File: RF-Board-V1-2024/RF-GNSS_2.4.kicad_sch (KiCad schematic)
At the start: 11 parts, among them J4 UART, J5 Conn_Coaxial, J7 Conn_Coaxial

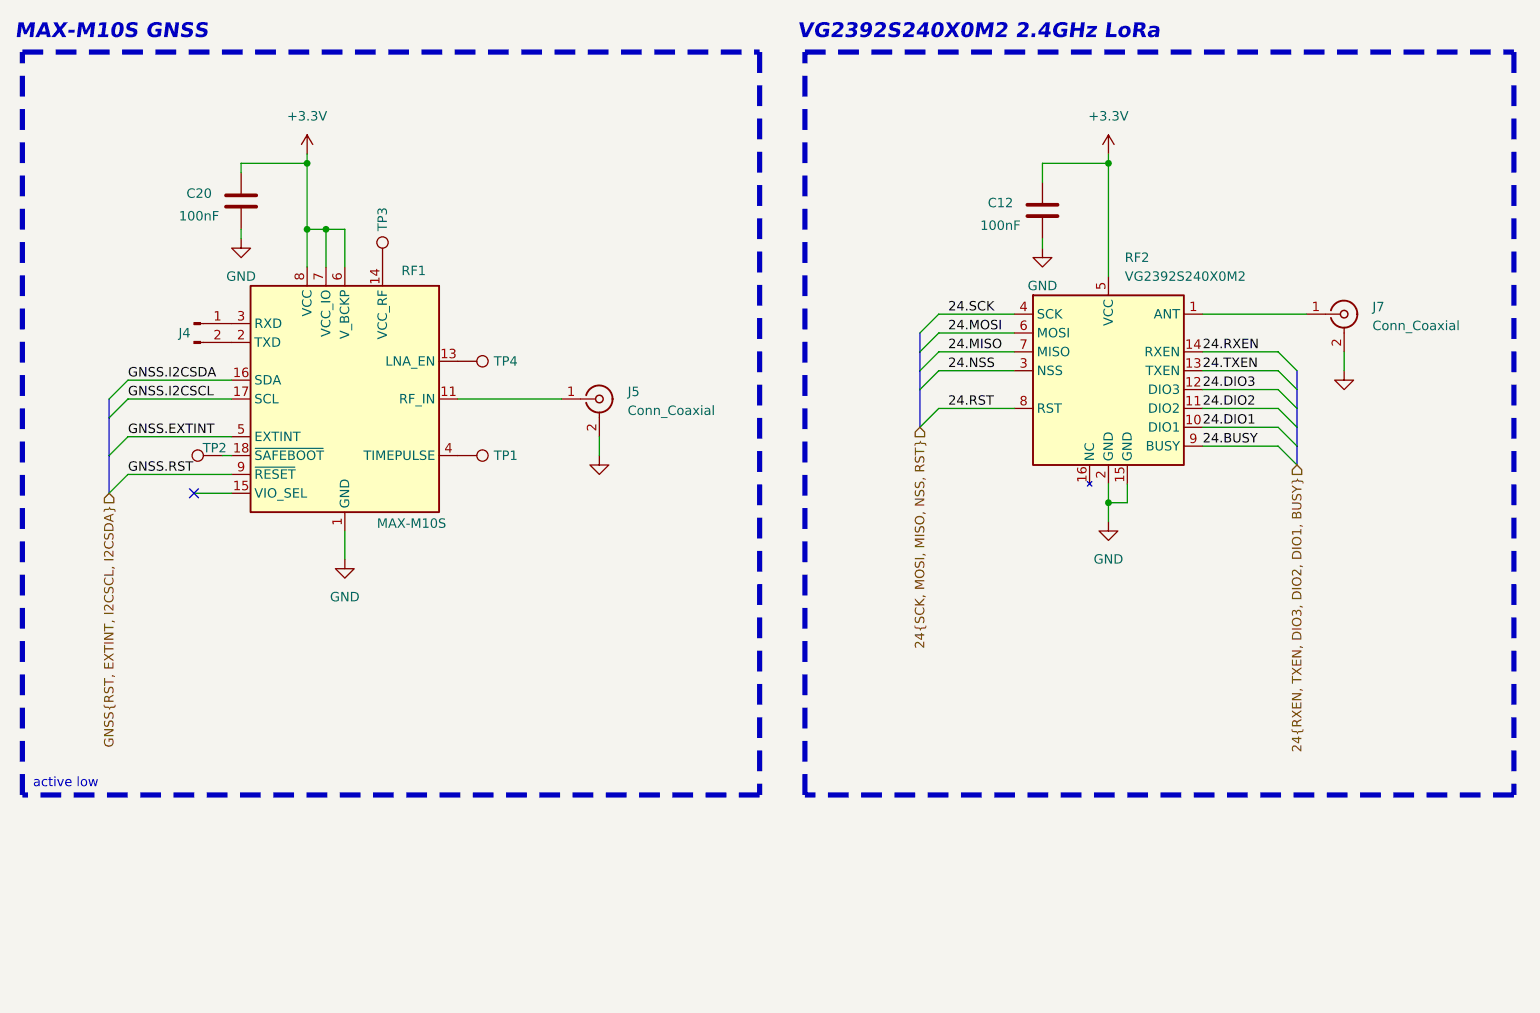
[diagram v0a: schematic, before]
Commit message: sd card need to do gnss
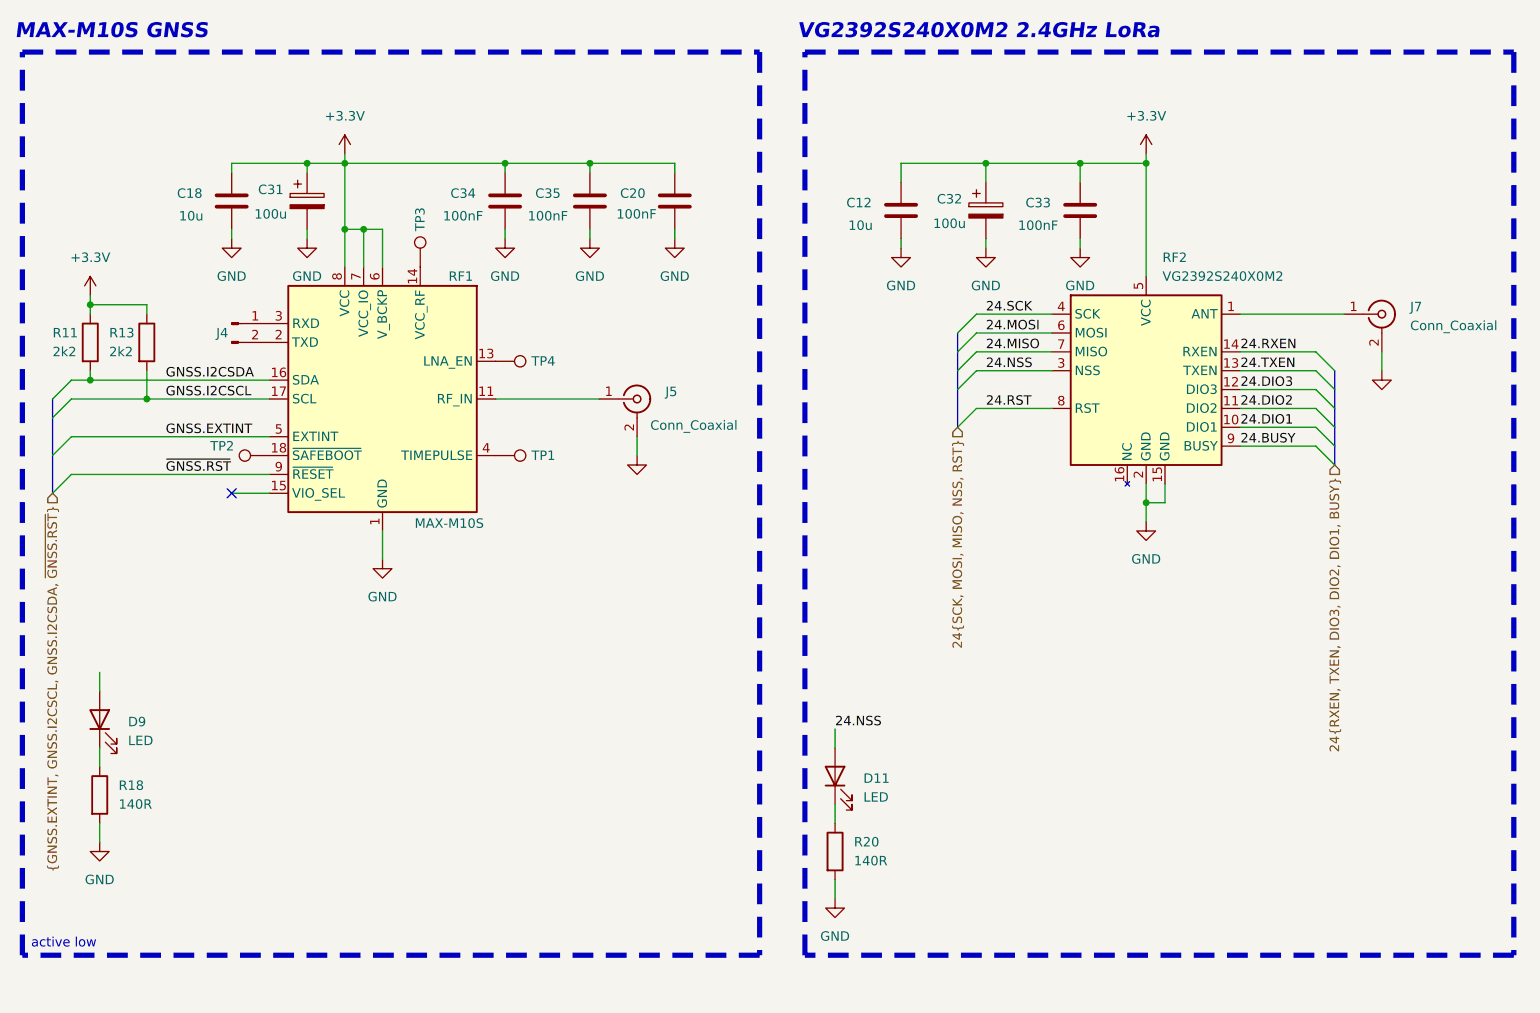
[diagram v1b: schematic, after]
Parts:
- added C18: 10u, symbol Device:C
- added C31, C32: 100u, Capacitor_SMD:CP_Elec_6.3x5.9, symbol Device:C_Polarized
- added C33, C34, C35: 100nF, symbol Device:C
- added D11, D9: LED, LED_SMD:LED_0603_1608Metric, symbol Device:LED
- added R11, R13: 2k2, Resistor_SMD:R_0603_1608Metric, symbol Device:R
- added R18, R20: 140R, Resistor_SMD:R_0603_1608Metric, symbol Device:R
- C12: value 100nF -> 10u
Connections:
- net +3.3V: now also C18.2, C31.1, C32.1, C33.2, C34.2, C35.2, R11.1, R13.1
- net 24.NSS: now also D11.2 (A)
- net GND: now also C18.1, C31.2, C32.2, C33.1, C34.1, C35.1, R18.2, R20.2
- net GNSS.I2CSCL: now also R13.2
- net GNSS.I2CSDA: now also R11.2
- net GNSS.RST renamed ~{GNSS.RST}
- new net: D9.1 (K), R18.1
- new net: D11.1 (K), R20.1
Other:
- moved on the sheet: J4, J5, J7, RF1, RF2, TP1, TP2, TP3, TP4
